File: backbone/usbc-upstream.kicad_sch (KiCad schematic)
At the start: 16 parts, among them J601 USB-C 24P receptacle, U601 HD3SS3220RNHR

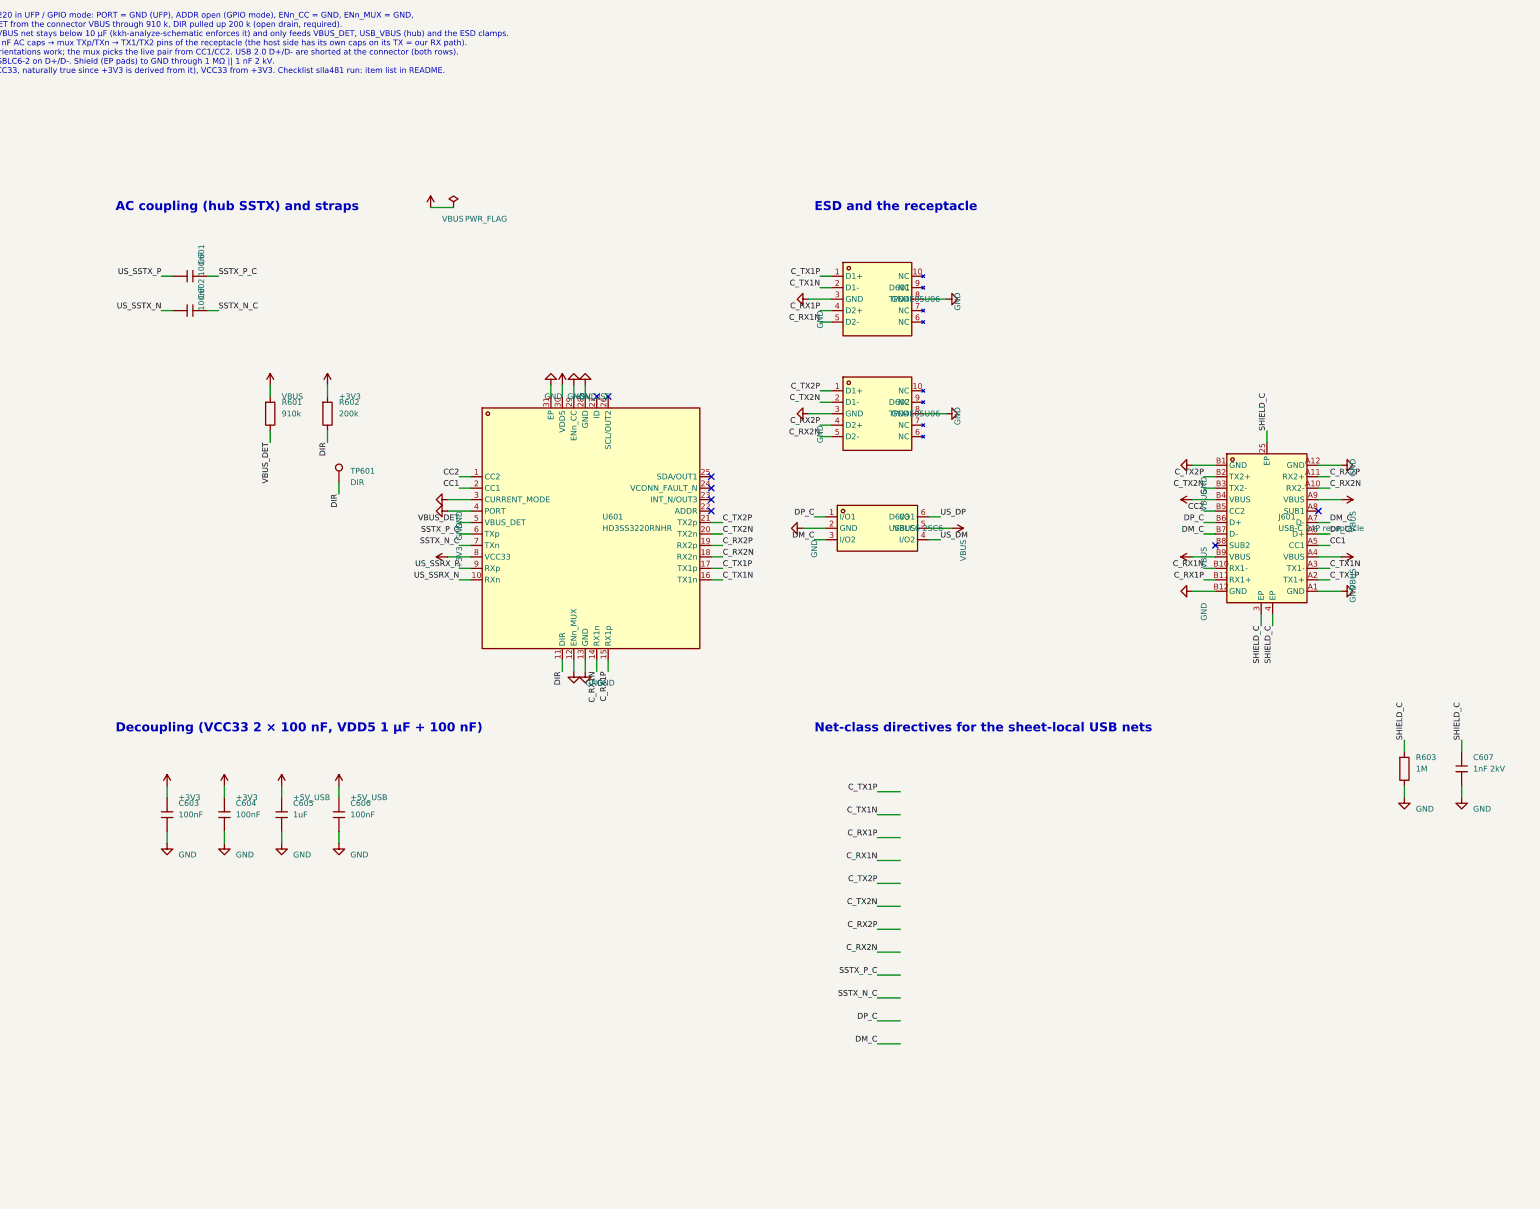
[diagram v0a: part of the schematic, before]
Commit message: schematics
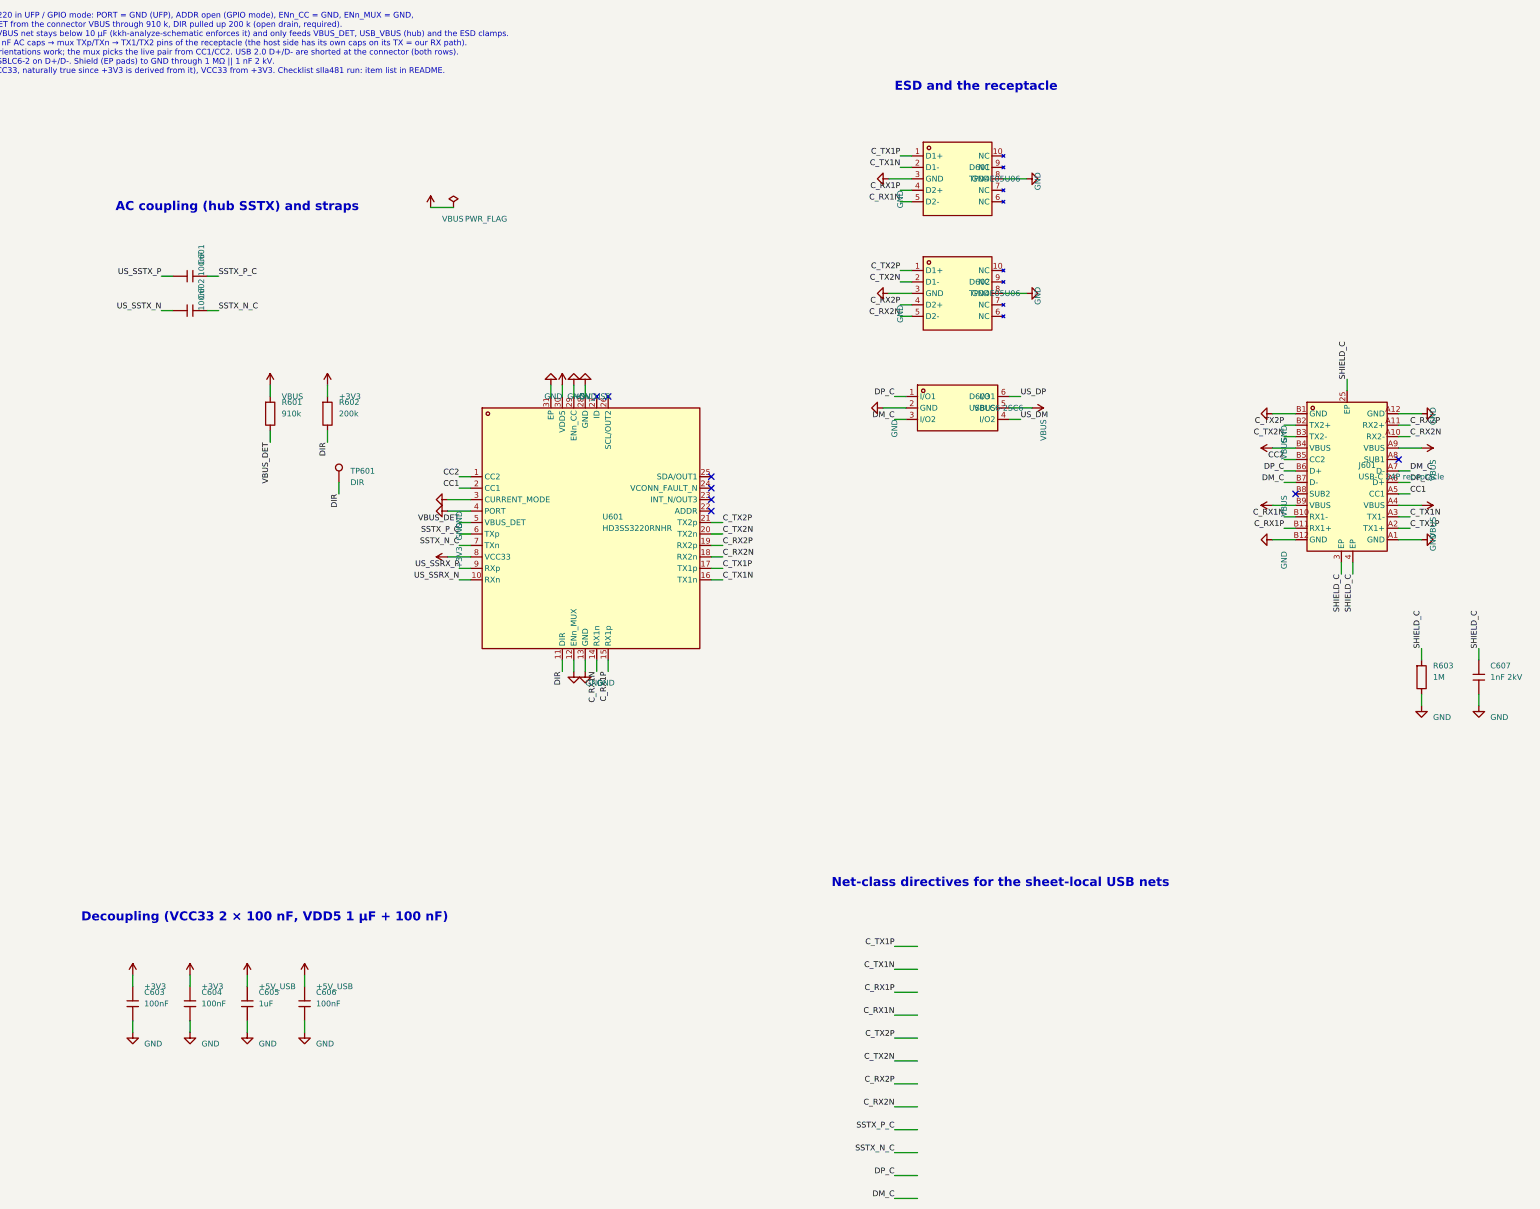
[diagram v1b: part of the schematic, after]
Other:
- moved on the sheet: C603, C604, C605, C606, C607, D601, D602, D603, J601, R603

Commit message: update
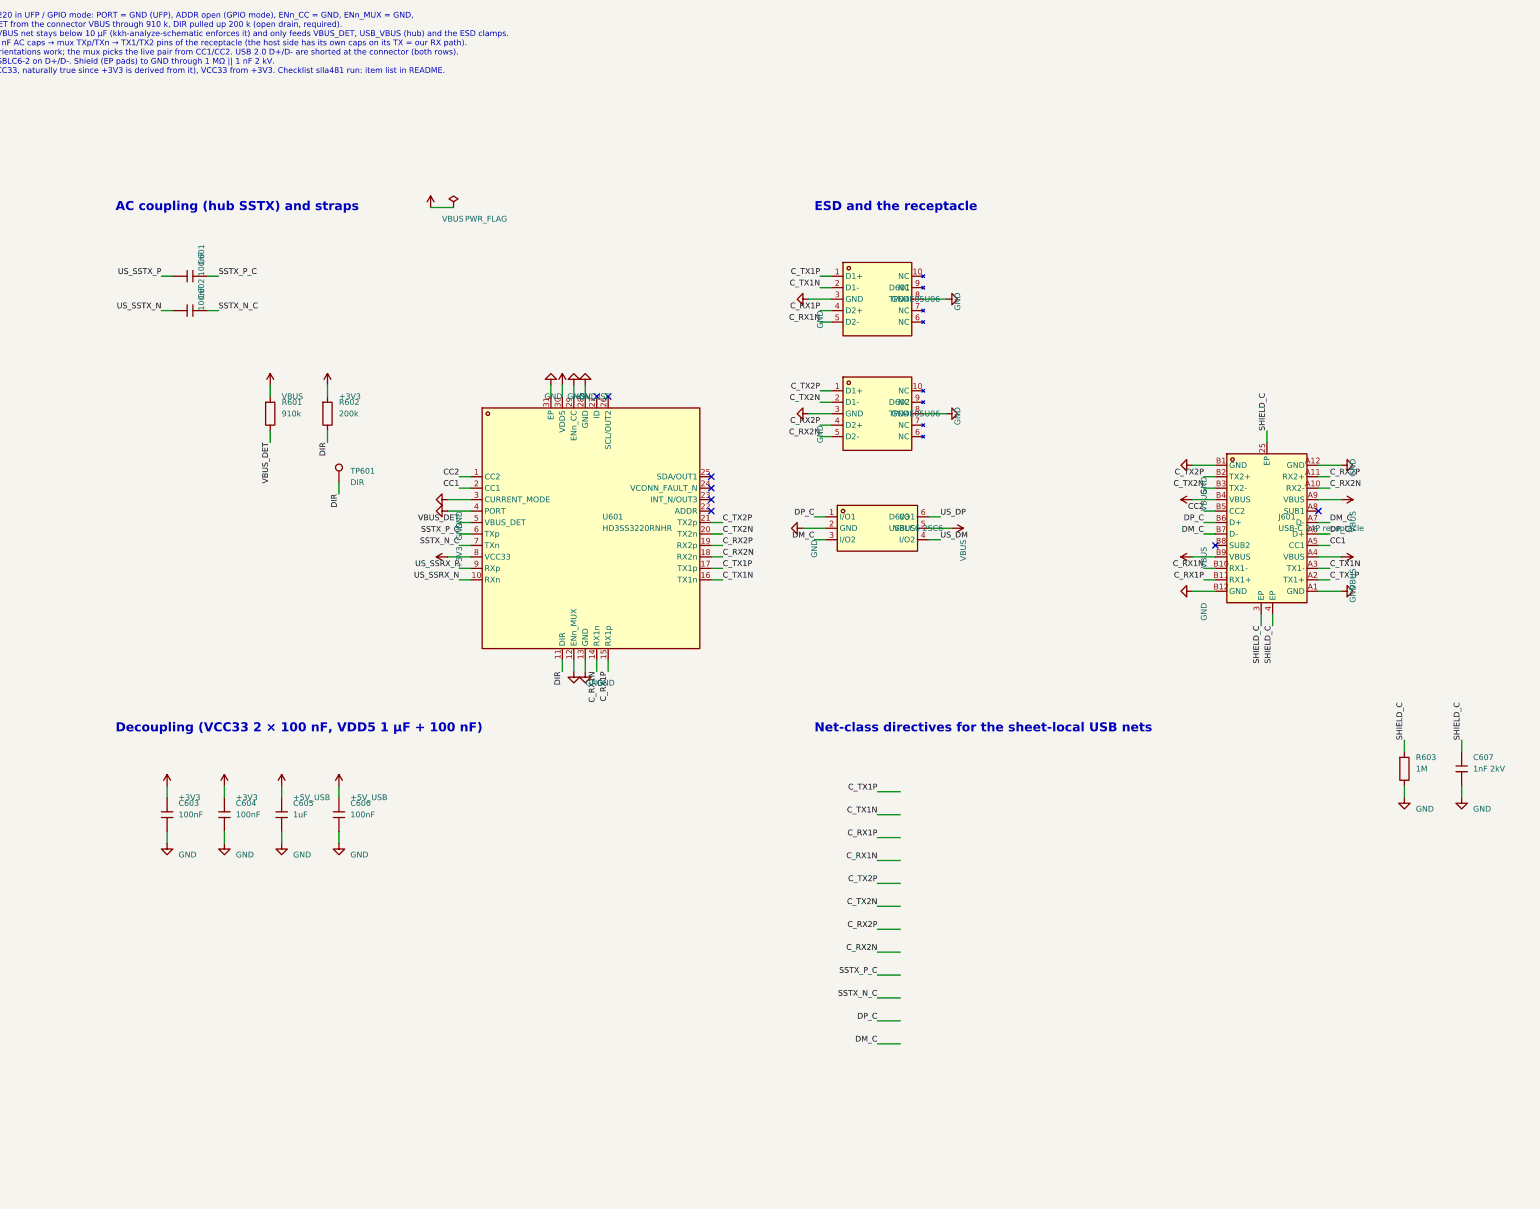
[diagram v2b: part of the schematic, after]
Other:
- moved on the sheet: C603, C604, C605, C606, C607, D601, D602, D603, J601, R603
